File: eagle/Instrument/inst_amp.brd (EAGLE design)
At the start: 53 x 40.6 mm, 12 parts, among them IC1 INA126U, X1 VCC +/-, X2 Vin, X3 Vout

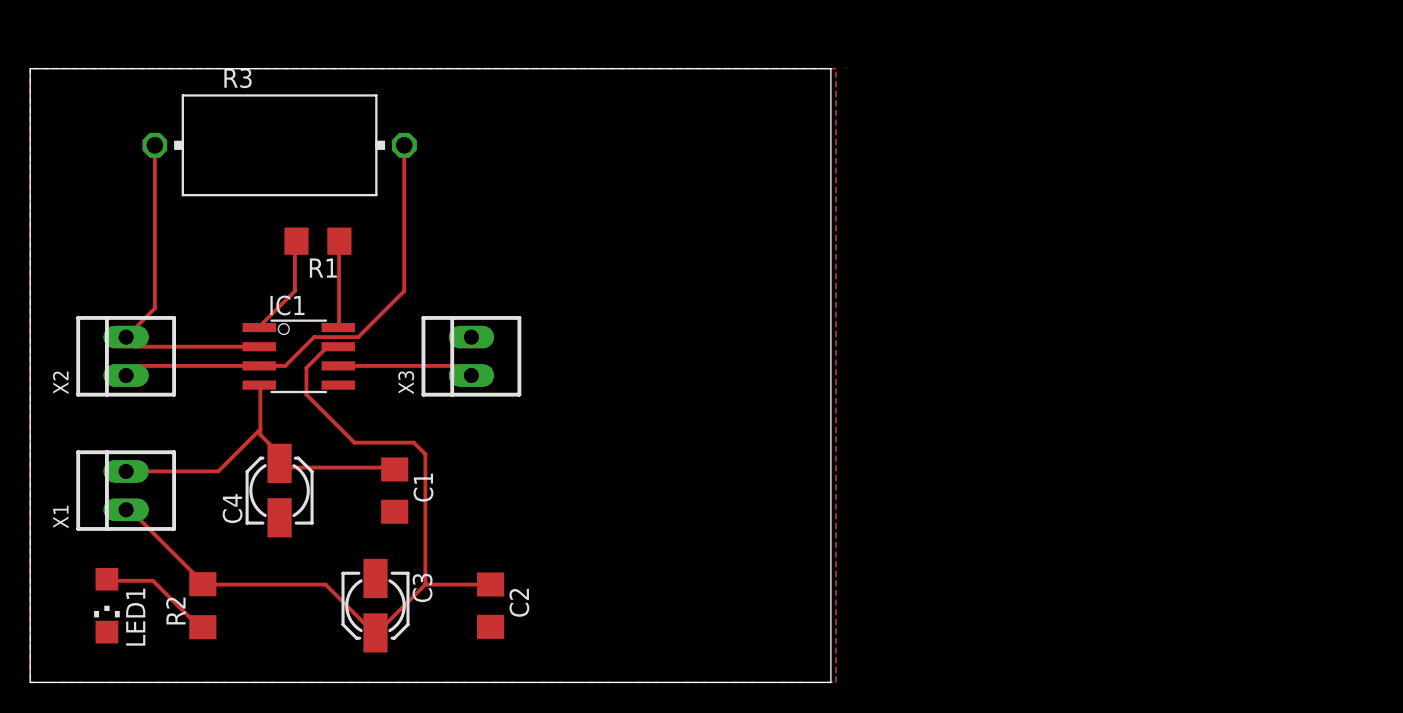
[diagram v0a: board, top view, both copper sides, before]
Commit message: PCB design done
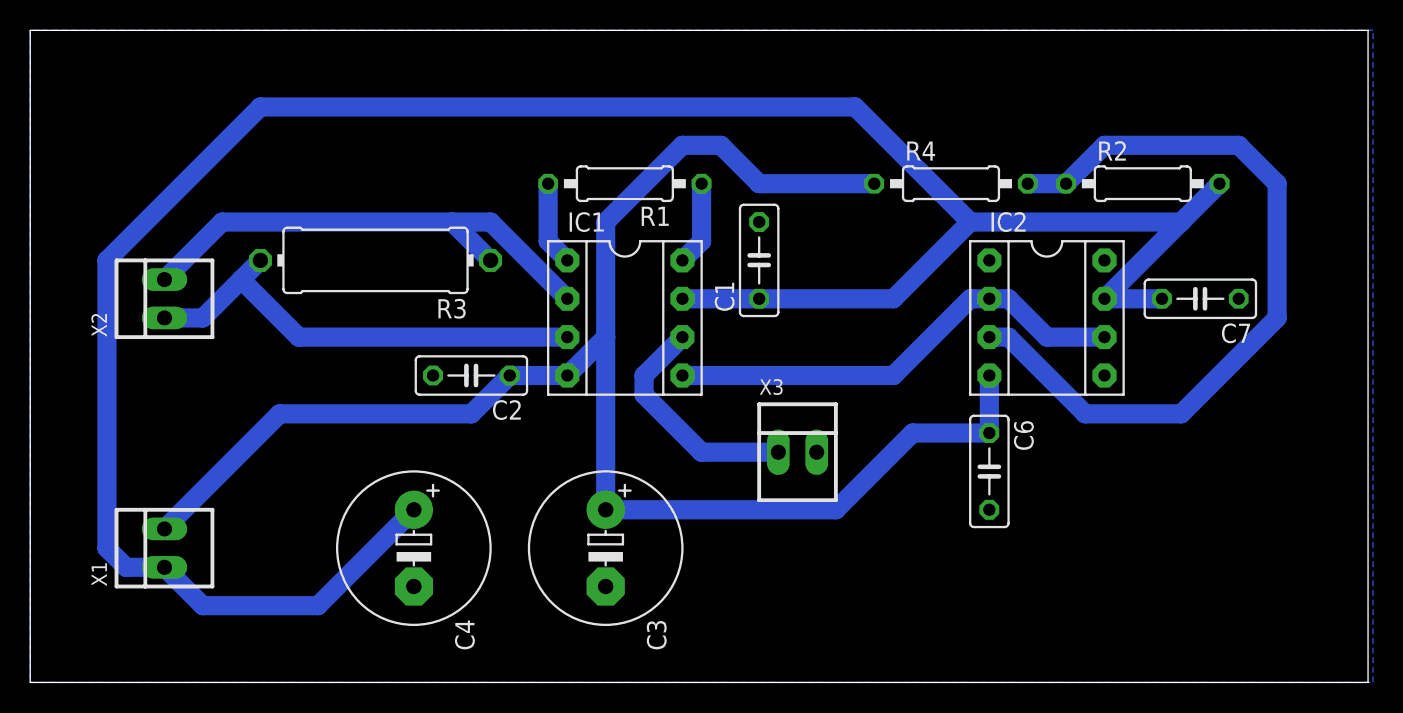
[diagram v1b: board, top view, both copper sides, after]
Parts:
- removed LED1: (no value), led:CHIPLED_1206
- added C6, C7: 100nF, rcl:C050-025X075
- added IC2: OP07C, burr-brown:DIL08
- added R4: 360R, rcl:0207/10
- C1, C2: device rcl:C1206 -> rcl:C050-025X075
- C3, C4: value 0,47µF -> 100µF; device rcl:153CLV-0405 -> rcl:E5-10,5
- IC1: value INA126U -> INA126P; device burr-brown:SO08 -> burr-brown:DIL08
- R1: value 18k -> 8k; device resistor:R1206 -> rcl:0207/10
- R2: value 330R -> 180R; device resistor:R1206 -> rcl:0207/10
- R3: value 0R33 -> 0R2; device rcl:VTA55 -> rcl:0414/15
- moved R2 68.2 mm to (73.7, 33.0), turned to 0 degrees
- moved C1 28.5 mm to (48.3, 27.9), turned to 90 degrees
- moved X3 22.5 mm to (50.8, 15.2), turned to 0 degrees
- moved IC1 21.7 mm to (39.4, 24.1)
- moved R1 20.7 mm to (39.4, 33.0)
- moved C3 15.7 mm to (38.1, 8.89)
- moved C2 15.3 mm to (29.2, 20.3), turned to 180 degrees
- moved R3 9.92 mm to (22.9, 27.9), turned to 180 degrees
- moved C4 9.67 mm to (25.4, 8.89), turned to 270 degrees
- moved X1 4.58 mm to (8.89, 8.89)
- moved X2 4.58 mm to (8.89, 25.4)
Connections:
- removed net N$3: C1.1, C4.+, IC1.4, X1.2
- removed net N$8: LED1.A, R2.1
- new net N$4: IC2.3, R2.1, R4.2
- new net REF: IC1.5, IC2.2, IC2.6
- new net V-: C2.1, C3.+, C6.1, IC1.4, IC2.4, R4.1, X1.2
- net GND: now also C6.2, C7.1; no longer LED1.C
- net V+: now also C1.1, C4.+, C7.2, IC2.7; no longer C2.1, C3.+
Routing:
- net V+: track 51.7 -> 157.8 mm
- net V-: track 0.00 -> 105.8 mm
- net N$4: track 0.00 -> 51.3 mm
- net REF: track 0.00 -> 31.1 mm
- net N$3: track 23.7 -> 0.00 mm
- net N$7: track 22.6 -> 33.9 mm
- net N$8: track 7.74 -> 0.00 mm
- net N$5: track 9.08 -> 15.3 mm
- net N$1: track 6.87 -> 5.61 mm
- net N$6: track 30.4 -> 31.1 mm
- removed copper zone on layer 1, net GND
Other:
- board size 53 x 40.6 mm -> 88.6 x 43.2 mm
